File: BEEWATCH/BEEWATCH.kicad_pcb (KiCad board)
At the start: 2 copper layers, 8 parts

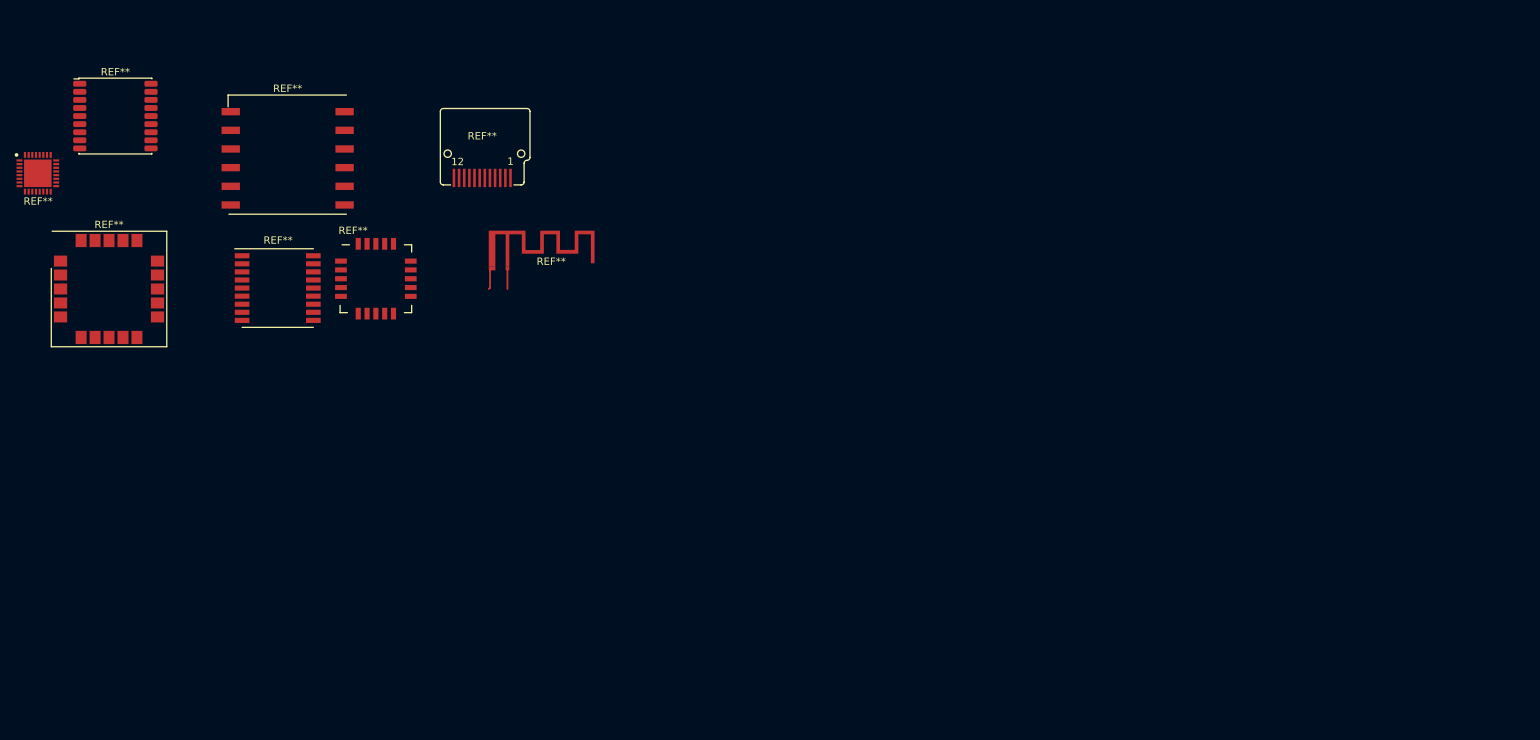
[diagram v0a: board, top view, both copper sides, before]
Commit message: Save Kicad files
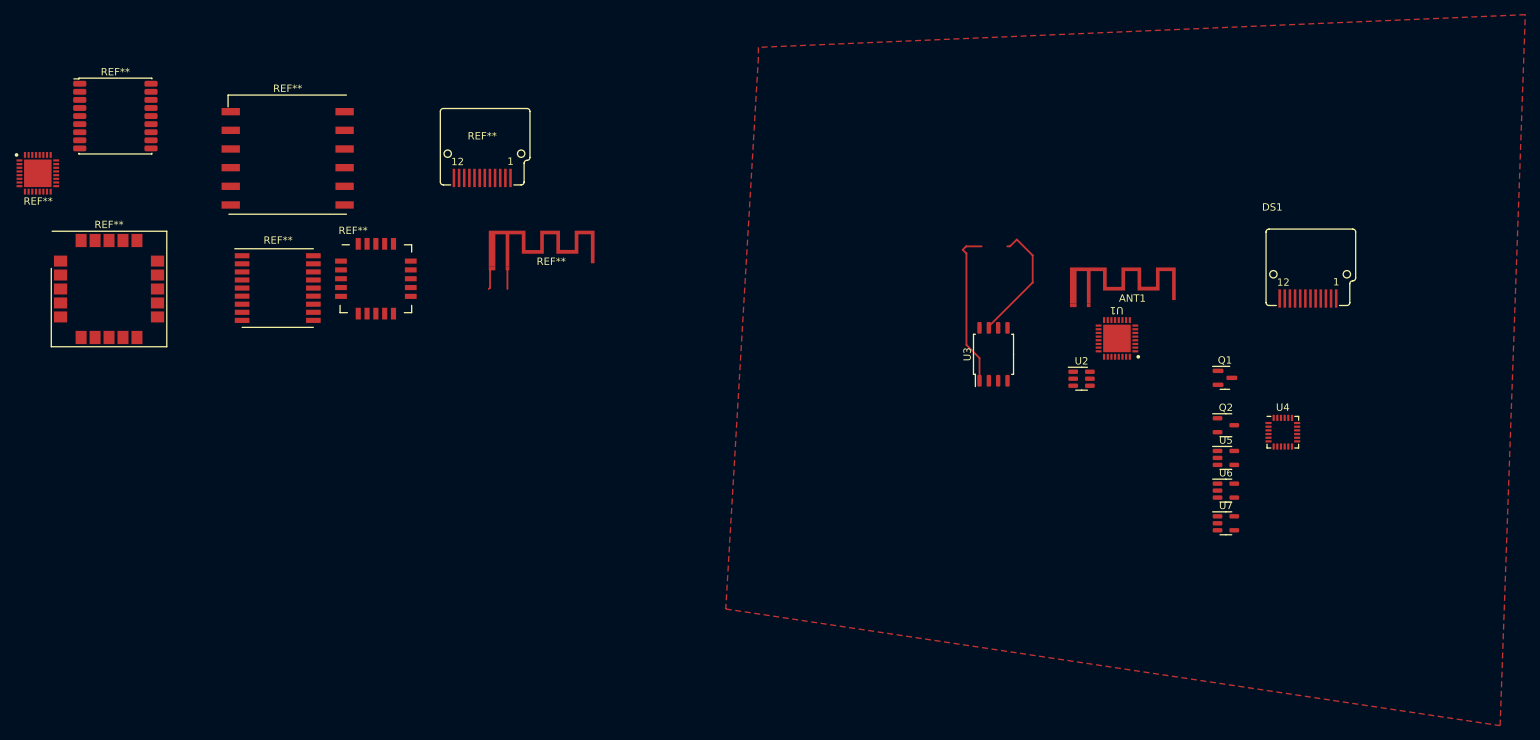
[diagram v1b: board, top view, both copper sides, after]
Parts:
- added ANT1: ~, Project:IFA_2.4GHz, F.Cu at (211.2, 63.4)
- added DS1: ~, Project:GC9A01_TOP, F.Cu at (243.8, 56.2)
- added Q1: 2N7002, Package_TO_SOT_SMD:SOT-23, F.Cu at (232.3, 73.1)
- added Q2: ~, Package_TO_SOT_SMD:SOT-23-3, F.Cu at (232.4, 79.5)
- added U1: ESP32-C3, Footprint:VFQFN-32, F.Cu at (217.6, 67.7)
- added U2: USBLC6-2SC6, Package_TO_SOT_SMD:SOT-23-6, F.Cu at (212.8, 73.2)
- added U3: W25Q128JVS, Package_SO:SOIC-8_5.23x5.23mm_P1.27mm, F.Cu at (200.8, 69.8)
- added U4: MPU-6050, Sensor_Motion:InvenSense_QFN-24_4x4mm_P0.5mm, F.Cu at (240.2, 80.5)
- added U5: MCP73832-2-OT, Package_TO_SOT_SMD:SOT-23-5, F.Cu at (232.4, 84.0)
- added U6: XC6210B332MR, Package_TO_SOT_SMD:SOT-23-5, F.Cu at (232.4, 88.4)
- added U7: XC6210B332MR, Package_TO_SOT_SMD:SOT-23-5, F.Cu at (232.4, 92.9)
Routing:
- net /ESP32/SPI2_CS0: track 0.00 -> 21.5 mm
- net /ESP32/SPI2_QUADHD: track 0.00 -> 17.1 mm
- added copper zone on F.Cu, net +5V
